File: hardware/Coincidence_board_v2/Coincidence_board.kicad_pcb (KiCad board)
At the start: 2 copper layers, 136.8 x 85 mm, 74 parts, among them J1 Inputs, J2 chan2_in, J3 POWER_IN, J4 Morpho_Gauche, J5 chan3_out, J7 Morpho_Droite, SW1 SW_1, U1 74HCT74, U2 74HCT74, U3 LM7805_TO220, U4 74HC74, U5 74HC74, U6 74HC74, U7 74HC74

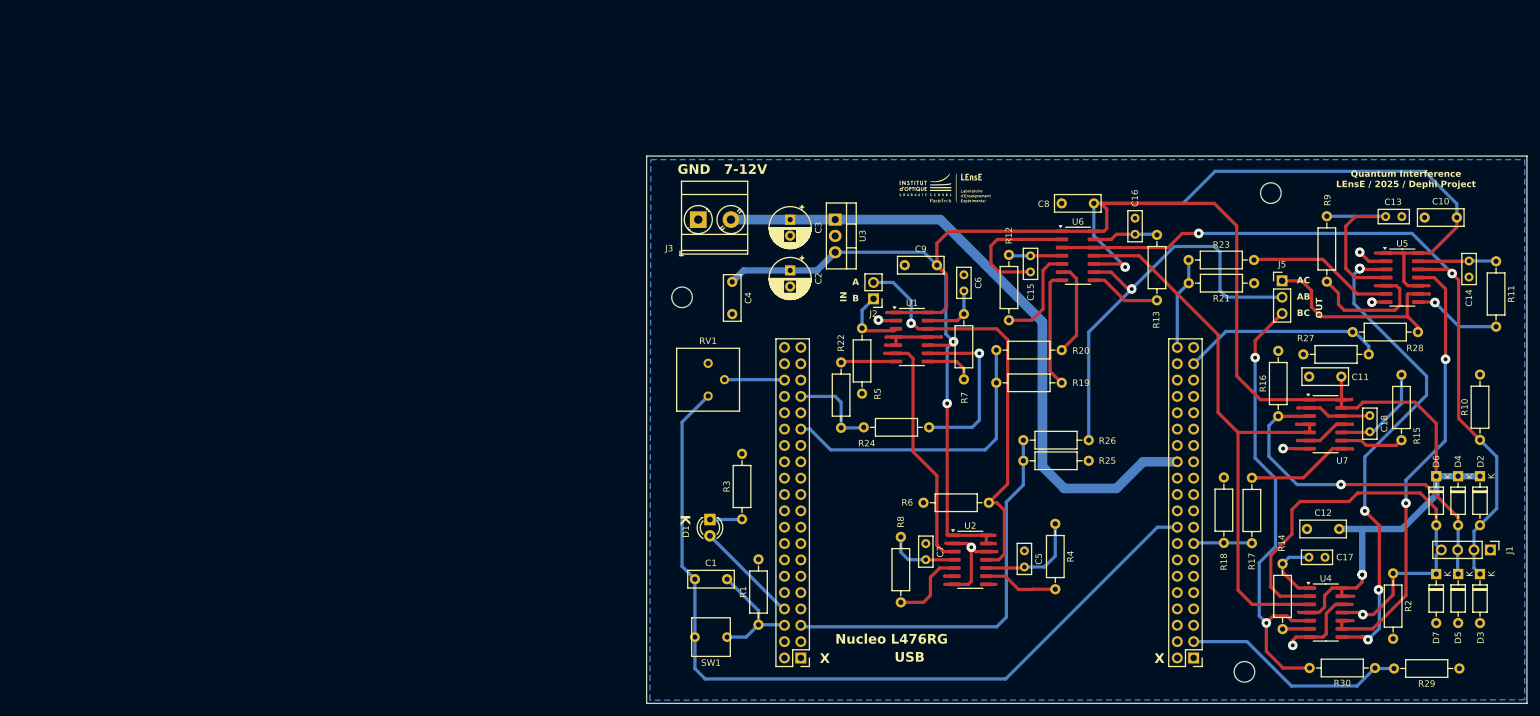
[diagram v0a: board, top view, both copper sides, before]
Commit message: Update Coincidence Board / v2
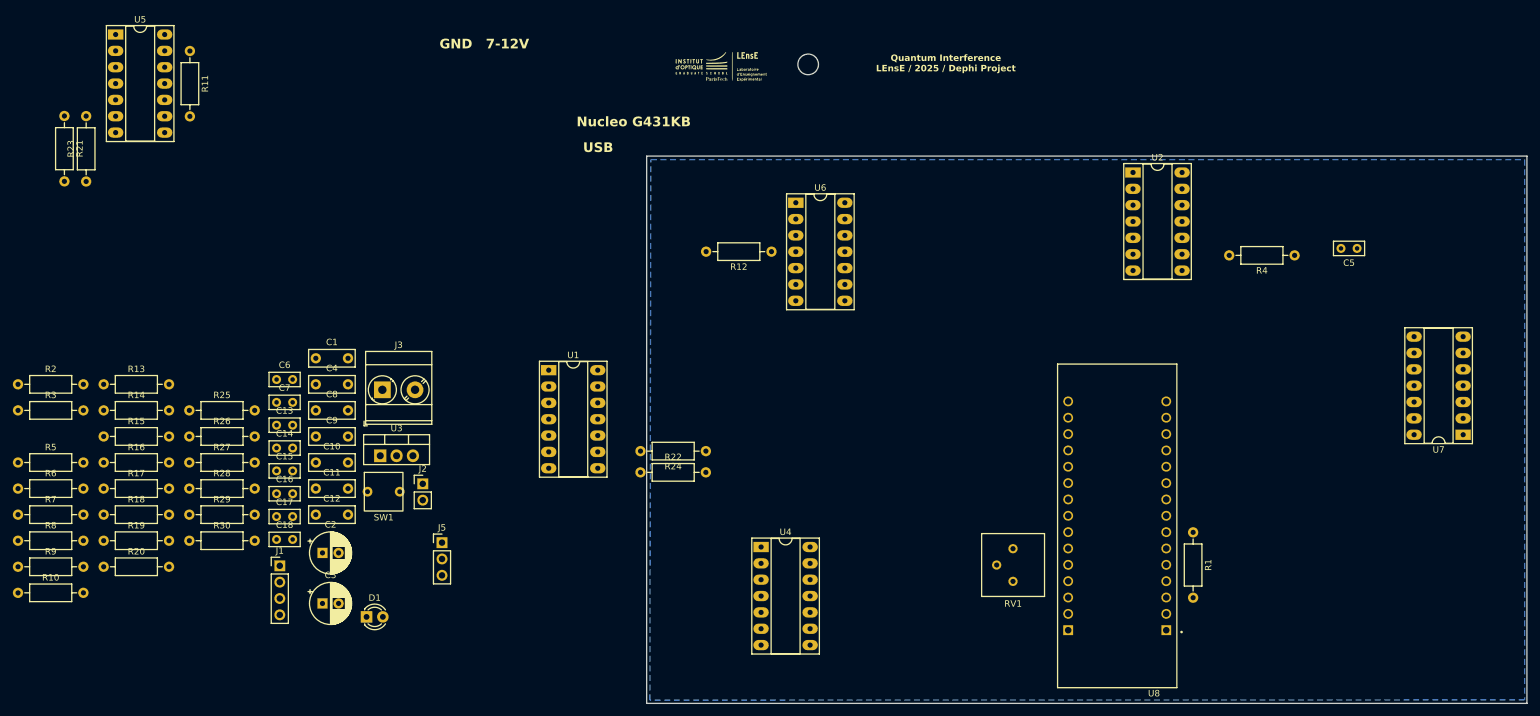
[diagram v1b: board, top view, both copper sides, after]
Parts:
- removed ? (x2): , 
- removed D2, D3, D4, D5, D6, D7: 1N4148, Diode_THT:D_DO-35_SOD27_P7.62mm_Horizontal
- removed J4: Morpho_Gauche, Connector_PinHeader_2.54mm:PinHeader_2x20_P2.54mm_Vertical
- removed J7: Morpho_Droite, Connector_PinHeader_2.54mm:PinHeader_2x20_P2.54mm_Vertical
- added U8: NUCLEO-L432KC, NUCLEO_L432KC:MODULE_NUCLEO-L432KC, F.Cu at (196.6, 122.9)
- U1, U2, U4, U5, U6, U7: footprint Package_SO:SO-14_3.9x8.65mm_P1.27mm -> Package_DIP:DIP-14_W7.62mm_Socket_LongPads
- moved R10 228.4 mm to (25.8, 133.3), turned to 0 degrees
- moved R2 215.7 mm to (25.8, 100.9), turned to 0 degrees
- moved R9 210.6 mm to (25.8, 129.3), turned to 0 degrees
- moved R11 205.6 mm to (52.5, 49.1)
- moved U5 203.5 mm to (41.0, 46.6)
- moved R15 201.9 mm to (39.1, 109.0), turned to 0 degrees
- moved R29 198.8 mm to (52.4, 121.2), turned to 0 degrees
- moved J1 188.1 mm to (66.5, 129.1), turned to 0 degrees
- moved C14 187.2 mm to (66.0, 110.8), turned to 0 degrees
- moved R21 186.7 mm to (33.0, 59.2), turned to -90 degrees
- moved R30 185.3 mm to (52.4, 125.2), turned to 0 degrees
- moved R14 184.7 mm to (39.1, 105.0), turned to 0 degrees
- moved R16 182.7 mm to (39.1, 113.1), turned to 0 degrees
- moved R28 182.4 mm to (52.4, 117.1)
- moved R17 178.6 mm to (39.1, 117.1), turned to 0 degrees
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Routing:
- net 5V: track 396.7 -> 0.00 mm, vias 5 -> 0
- net 3.3V_NUC: track 130.3 -> 0.00 mm
- net A2in: track 121.0 -> 0.00 mm, vias 2 -> 0
- net GND: track 105.8 -> 0.00 mm, vias 6 -> 0
- net VIN: track 101.6 -> 0.00 mm
- net Net-(U4A-C): track 91.9 -> 0.00 mm
- net Net-(U4B-~{Q}): track 77.7 -> 0.00 mm, vias 5 -> 0
- net C2in: track 74.8 -> 0.00 mm, vias 1 -> 0
- net BC2out: track 72.4 -> 0.00 mm, vias 2 -> 0
- net Net-(U4B-Q): track 70.4 -> 0.00 mm, vias 2 -> 0
- net AB2out: track 66.1 -> 0.00 mm, vias 1 -> 0
- net Ain: track 66.1 -> 0.00 mm, vias 1 -> 0
- net AB2out_nuc: track 61.3 -> 0.00 mm
- net B2in: track 53.9 -> 0.00 mm, vias 1 -> 0
- net A2out_nuc: track 46.2 -> 0.00 mm
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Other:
- board text added: "Nucleo G431KB"
- board text removed: "A"
- board text removed: "AB"
- board text removed: "AC"
- board text removed: "B"
- board text removed: "BC"
- board text removed: "IN"
- board text removed: "K"
- board text removed: "Nucleo L476RG"
- board text removed: "OUT"
- board text removed: "X"
